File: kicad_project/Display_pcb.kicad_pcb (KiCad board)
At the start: 4 copper layers, 60.6 x 27.6 mm, 89 parts, among them IC1 ESP32-S3R8, J1 Micro_SD_Card_Det_Hirose_DM3AT, J2 USB C, J8 33FXRH-SM1-GAN-TF, Q1 S8050, Q2 BSS84, Q3 S8050, SW1 B3U-1000P, SW2 B3U-1000P, SW3 B3U-1000P, U1 W25Q128JVSIQ, U2 SY8089A1AAC, U3 AXPM65611, U5 USBLC6-2SC6, Y1 40MHz

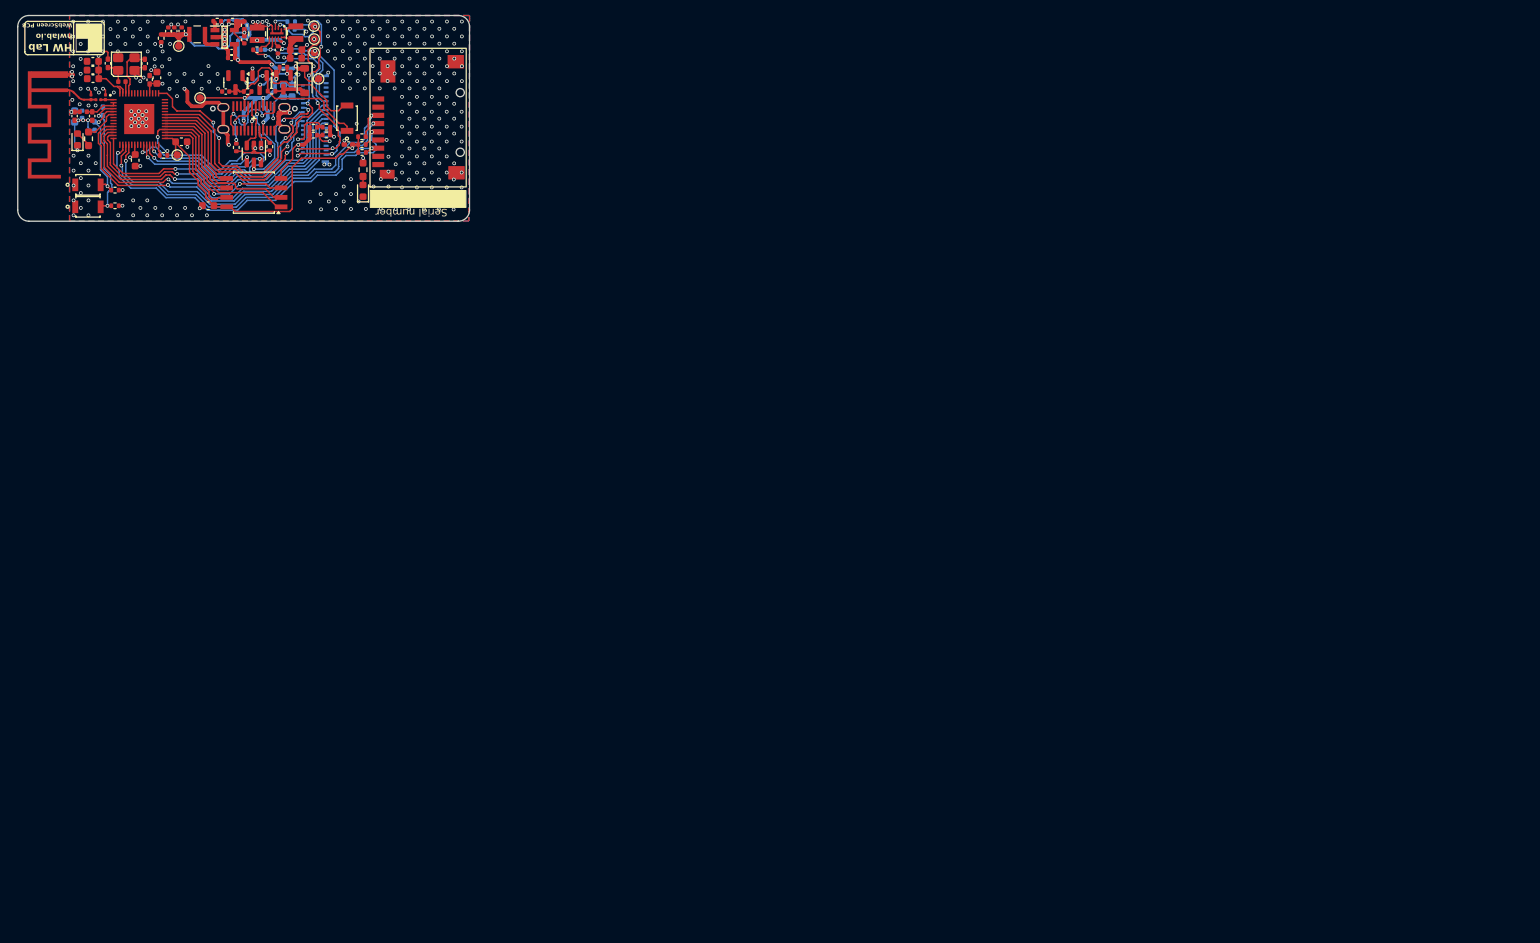
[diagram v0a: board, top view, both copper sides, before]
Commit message: Pcb to production
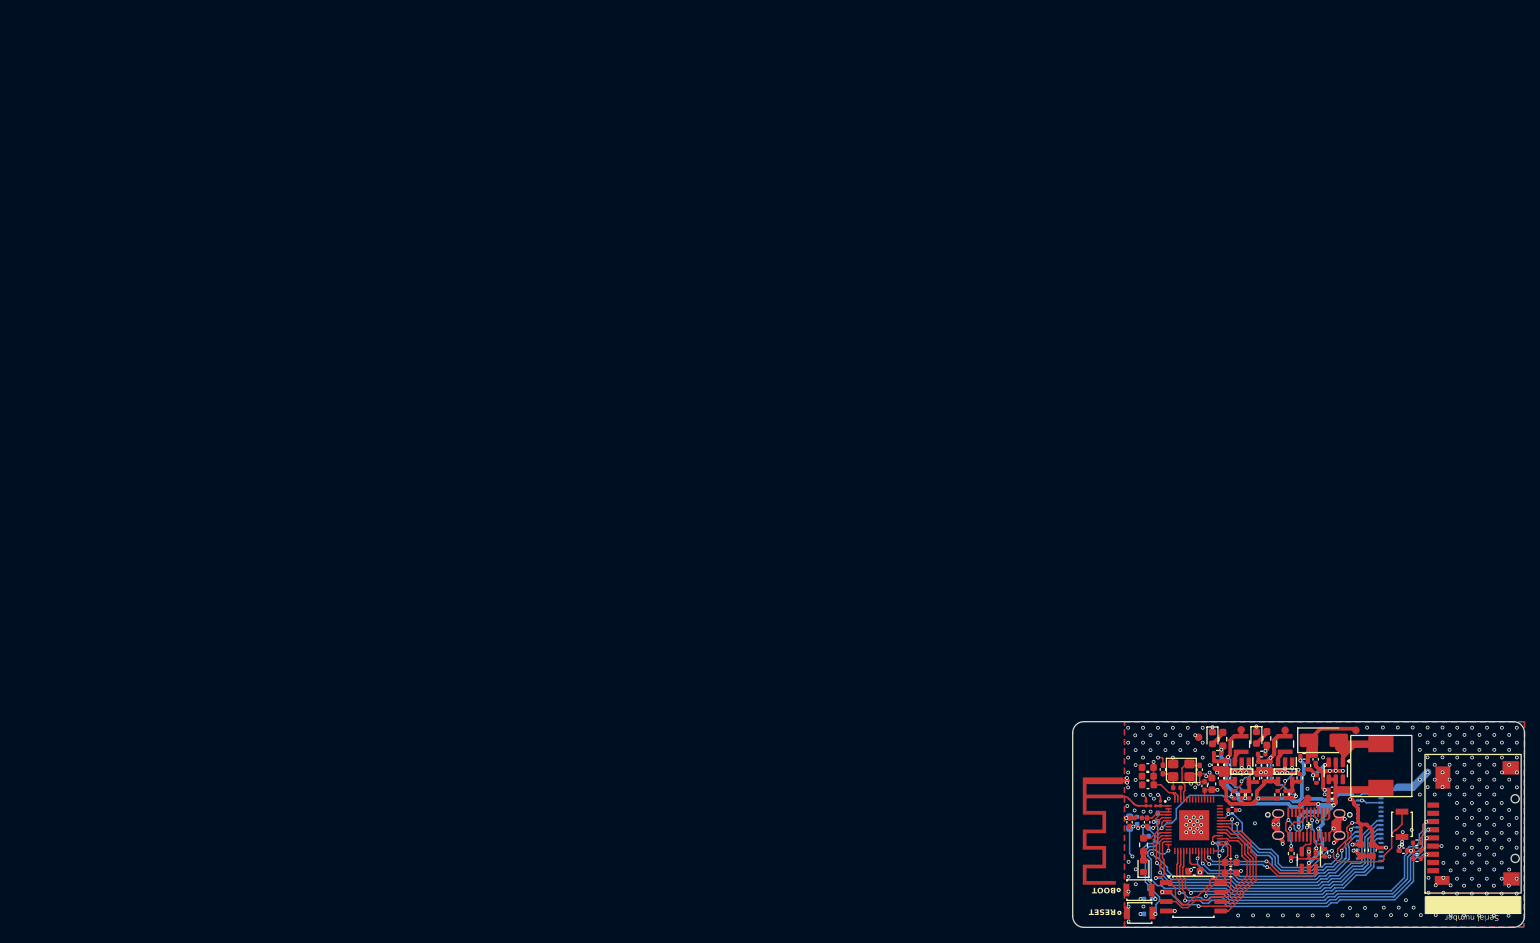
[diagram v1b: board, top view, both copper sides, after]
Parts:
- removed D2: B5819W, Diode_SMD:D_SOD-123
- removed L7, L8: DFP252012TF-100M, smd-non-ipc:DFE252012P-1R0M=P2
- removed Q1, Q3: S8050, Package_TO_SOT_SMD:SOT-23
- removed Q2: BSS84, Package_TO_SOT_SMD:SOT-23
- removed R22: TBD, Resistor_SMD:R_0402_1005Metric
- removed R30: 100k, Resistor_SMD:R_0402_1005Metric
- removed R31: 680k, Resistor_SMD:R_0402_1005Metric
- removed TP6: VDD_SPI, TestPoint:TestPoint_Pad_D1.0mm
- removed TP7: +5V, TestPoint:TestPoint_Pad_D1.0mm
- added C34: 22uF, Capacitor_SMD:C_0402_1005Metric, F.Cu at (144.6, 92.1)
- added C35: 100nF, Capacitor_SMD:C_0402_1005Metric, F.Cu at (143.8, 92.1)
- added C36: 22uF, Capacitor_SMD:C_0402_1005Metric, F.Cu at (143.0, 92.1)
- added C37: 22uF, Capacitor_SMD:C_0402_1005Metric, F.Cu at (152.8, 95.4)
- added D1: SS34, Diode_SMD:D_SMA, F.Cu at (151.8, 88.8)
- added DS3: GREEN, LED_SMD:LED_0603_1608Metric, F.Cu at (142.7, 88.4)
- added G***: LOGO, logo:OSHWA_Certification.kicad_sym, B.Cu at (169.8, 106.8)
- added L4: 1uH, smd-non-ipc:BR2518_YDN, F.Cu at (146.6, 89.2)
- added L6: 22uH, smd-non-ipc:MDA7030-220M, F.Cu at (159.4, 92.4)
- added NT1: NetTie_2, NetTie:NetTie-2_SMD_Pad0.5mm, F.Cu at (158.2, 101.3)
- added NT2: NetTie_2, NetTie:NetTie-2_SMD_Pad0.5mm, F.Cu at (156.7, 101.3)
- added R17: 22k, Resistor_SMD:R_0402_1005Metric, F.Cu at (148.5, 93.8)
- added R18: 0R, Resistor_SMD:R_0402_1005Metric, F.Cu at (143.4, 90.6)
- added R23: 1k, Resistor_SMD:R_0603_1608Metric_Pad0.98x0.95mm_HandSolder, F.Cu at (144.1, 88.5)
- added U4: SY8089A1AAC, smd-non-ipc:SOT95P285X130-5N, F.Cu at (146.6, 93.0)
- C18, C30: value 10uF -> 22uF
- C27: value 10uF -> 22uF; moved to F.Cu
- C28: value 1uF -> 22uF; footprint Capacitor_SMD:C_0603_1608Metric -> Capacitor_SMD:C_0402_1005Metric
- C29: value 1uF -> 100nF; footprint Capacitor_SMD:C_0603_1608Metric -> Capacitor_SMD:C_0402_1005Metric
- C31: value 10uF -> 6.8pF; moved to F.Cu
- C32, C33: moved to F.Cu
- G***, R1, R2, R8: moved to B.Cu
- J2: footprint hwlab:USB_C_Receptacle_HCTL_HC019-1E1H1A103-0HR -> paltatech:USB_C_Receptacle_HCTL_HC019-1E1H1A103-0HR
- R10: value 22k -> 10k
- R13: value 0R -> 100k
- R14: value 0R -> 100k; moved to F.Cu
- R20: value 0R -> 10k
- R21: value 0R -> 80k6
- R7: value 100k -> 10k
- R9: value 100k -> 64k9
- SW1, SW2, SW3: footprint hwlab:B3U-1000P -> smd-non-ipc:B3U-1000P
- TP2: value +3V3 -> +4V6
- TP3: value +4V6 -> +5V4
- TP4: value -2V2 -> +3V3
- U3: value AXPM65611 -> MT3608; footprint smd-non-ipc:DFN-12 -> Package_TO_SOT_SMD:SOT-23-6
- moved G*** 220.4 mm to (173.8, 110.0), turned to 90 degrees
- moved C32 177.2 mm to (158.2, 103.5), turned to -90 degrees
- moved C33 176.8 mm to (156.7, 103.5), turned to -90 degrees
- moved TP1 175.9 mm to (149.6, 96.5)
- moved C27 175.6 mm to (152.8, 97.0)
- moved DS1 173.1 mm to (127.5, 105.7)
- moved U3 172.6 mm to (153.3, 92.8), turned to -90 degrees
- moved C14 171.6 mm to (139.2, 106.5)
- moved C18 171.5 mm to (150.7, 91.3), turned to -90 degrees
- moved C23 171.5 mm to (137.9, 92.0), turned to -90 degrees
- moved C24 171.5 mm to (137.1, 92.0), turned to -90 degrees
- moved R11 171.4 mm to (139.7, 96.0), turned to -90 degrees
- moved C22 171.4 mm to (138.8, 92.0), turned to -90 degrees
- moved R32 171.2 mm to (137.5, 90.5), turned to 0 degrees
- moved C15 171.1 mm to (134.3, 106.3), turned to 180 degrees
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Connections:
- C18 pad 1: Net-(Q3-C) -> Net-(D1-K)
- C27 pad 1: EAVDD -> /POWER/VBUS
- C28 pad 1: +3V3 -> /POWER/VBUS
- C29 pad 1: +3V3 -> VCC
- C30 pad 1: -2V2 -> VCC
- C31 pad 1: 4.6V -> Net-(C31-Pad1)
- C31 pad 2: GND -> Net-(U4-FB)
- C32 pad 1: +3V3 -> /AVDD
- C33 pad 1: +3V3 -> Net-(J8-Pin_26)
- IC1 pad 38: unconnected-(IC1-GPIO33-Pad38) -> /MCU/GPIO33
- IC1 pad 43: /OL_EN -> /GPIO38
- J2 pad A4: VBUS -> /POWER/VBUS
- J2 pad A9: VBUS -> /POWER/VBUS
- J2 pad B4: VBUS -> /POWER/VBUS
- J2 pad B9: VBUS -> /POWER/VBUS
- J8 pad 1: unconnected-(J8-Pin_1-Pad1) -> GND
- J8 pad 10: /OL_EN -> unconnected-(J8-Pin_10-Pad10)
- J8 pad 11: /OL_TE -> unconnected-(J8-Pin_11-Pad11)
- J8 pad 12: /OL_RESET -> unconnected-(J8-Pin_12-Pad12)
- J8 pad 13: /OL_SD0 -> unconnected-(J8-Pin_13-Pad13)
- J8 pad 14: /OL_D0 -> unconnected-(J8-Pin_14-Pad14)
- J8 pad 15: /OL_D1 -> /OL_D3
- J8 pad 16: /OL_SCK -> /OL_D2
- J8 pad 18: /OL_D2 -> /OL_SCK
- J8 pad 19: /OL_D3 -> /OL_D1
- J8 pad 2: unconnected-(J8-Pin_2-Pad2) -> GND
- J8 pad 20: unconnected-(J8-Pin_20-Pad20) -> /OL_D0
- J8 pad 21: unconnected-(J8-Pin_21-Pad21) -> /OL_SD0
- J8 pad 22: unconnected-(J8-Pin_22-Pad22) -> /OL_RESET
- J8 pad 23: unconnected-(J8-Pin_23-Pad23) -> /OL_TE
- J8 pad 26: /IM1 -> Net-(J8-Pin_26)
- J8 pad 27: /IM0 -> /AVDD
- J8 pad 3: unconnected-(J8-Pin_3-Pad3) -> 4.6V
- J8 pad 30: 4.6V -> unconnected-(J8-Pin_30-Pad30)
- J8 pad 31: 4.6V -> unconnected-(J8-Pin_31-Pad31)
- J8 pad 32: -2V2 -> unconnected-(J8-Pin_32-Pad32)
- J8 pad 33: -2V2 -> unconnected-(J8-Pin_33-Pad33)
- J8 pad 4: unconnected-(J8-Pin_4-Pad4) -> 4.6V
- J8 pad 7: EAVDD -> GND
- J8 pad 9: /SWIRE -> unconnected-(J8-Pin_9-Pad9)
- R11 pad 2: VCC -> /MCU/GPIO1
- R13 pad 1: Net-(U3-CTRL) -> Net-(U4-EN)
- R13 pad 2: /SWIRE -> VCC
- R14 pad 1: Net-(U3-EN) -> Net-(C31-Pad1)
- R14 pad 2: /OL_EN -> Net-(U4-FB)
- R16 pad 2: +3V3 -> 4.6V
- R19 pad 1: /IM1 -> Net-(D1-K)
- R19 pad 2: +3V3 -> VCC
- R20 pad 1: /IM0 -> Net-(U3-FB)
- R20 pad 2: +3V3 -> GND
- R21 pad 1: GND -> Net-(D1-K)
- R21 pad 2: /IM0 -> Net-(U3-FB)
- R32 pad 2: +3V3 -> 4.6V
- R7 pad 1: VBUS -> +3V3
- R7 pad 2: Net-(Q1-C) -> /MCU/GPIO33
- SW3 pad 1: Net-(Q1-B) -> GND
- SW3 pad 2: Net-(Q3-C) -> /MCU/GPIO33
- TP1 pad 1: VBUS -> /POWER/VBUS
- TP3 pad 1: 4.6V -> Net-(D1-K)
- TP4 pad 1: -2V2 -> Net-(C31-Pad1)
- U3 pad 3: 4.6V -> Net-(U3-FB)
- U3 pad 4: Net-(U3-EN) -> /POWER/VBUS
- U3 pad 5: GND -> /POWER/VBUS
- U5 pad 5: VBUS -> /POWER/VBUS
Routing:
- net /OL_EN: track 51.9 -> 0.00 mm, vias 5 -> 0
- net /POWER/VBUS: track 0.00 -> 47.9 mm, vias 0 -> 5
- net VBUS: track 38.0 -> 0.00 mm, vias 6 -> 0
- net /MCU/GPIO33: track 0.00 -> 36.6 mm, vias 0 -> 2
- net GND: track 104.2 -> 135.7 mm, vias 333 -> 291
- net Net-(D1-A): track 1.75 -> 31.7 mm
- net -2V2: track 29.0 -> 0.00 mm, vias 4 -> 0
- net Net-(C31-Pad1): track 0.00 -> 28.1 mm, vias 0 -> 2
- net Net-(Q3-C): track 22.2 -> 0.00 mm
- net Net-(Q1-B): track 20.5 -> 0.00 mm, vias 2 -> 0
- net Net-(D1-K): track 0.00 -> 20.3 mm
- net /SWIRE: track 16.1 -> 0.00 mm, vias 1 -> 0
- net EAVDD: track 15.6 -> 0.00 mm, vias 1 -> 0
- net /MCU/GPIO1: track 4.61 -> 17.1 mm, vias 0 -> 2
- net +3V3: track 41.3 -> 29.0 mm, vias 11 -> 9
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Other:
- board text added: "BOOT"
- board text added: "DISPLAY"
- board text added: "RESET"
